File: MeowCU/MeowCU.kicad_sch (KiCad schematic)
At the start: 66 parts, among them J1 SWD, J10 Screw_Terminal_01x03, J11 Conn_02x10_Odd_Even, J2 Conn_02x04_Odd_Even, J4 SPI1, J5 5V_IN, J6 OLED, J7 USB_C_Receptacle_USB2.0_16P, J9 PWM, SW1 SW_SPST, SW6 BTN_UTIL, SW8 BTN_UTIL, SW9 BTN_UTIL, U1 STM32F405RGT6, U2 USBLC6-2SC6, U3 SN65HVD230, U4 AP2112K-3.3, Y1 25MHz

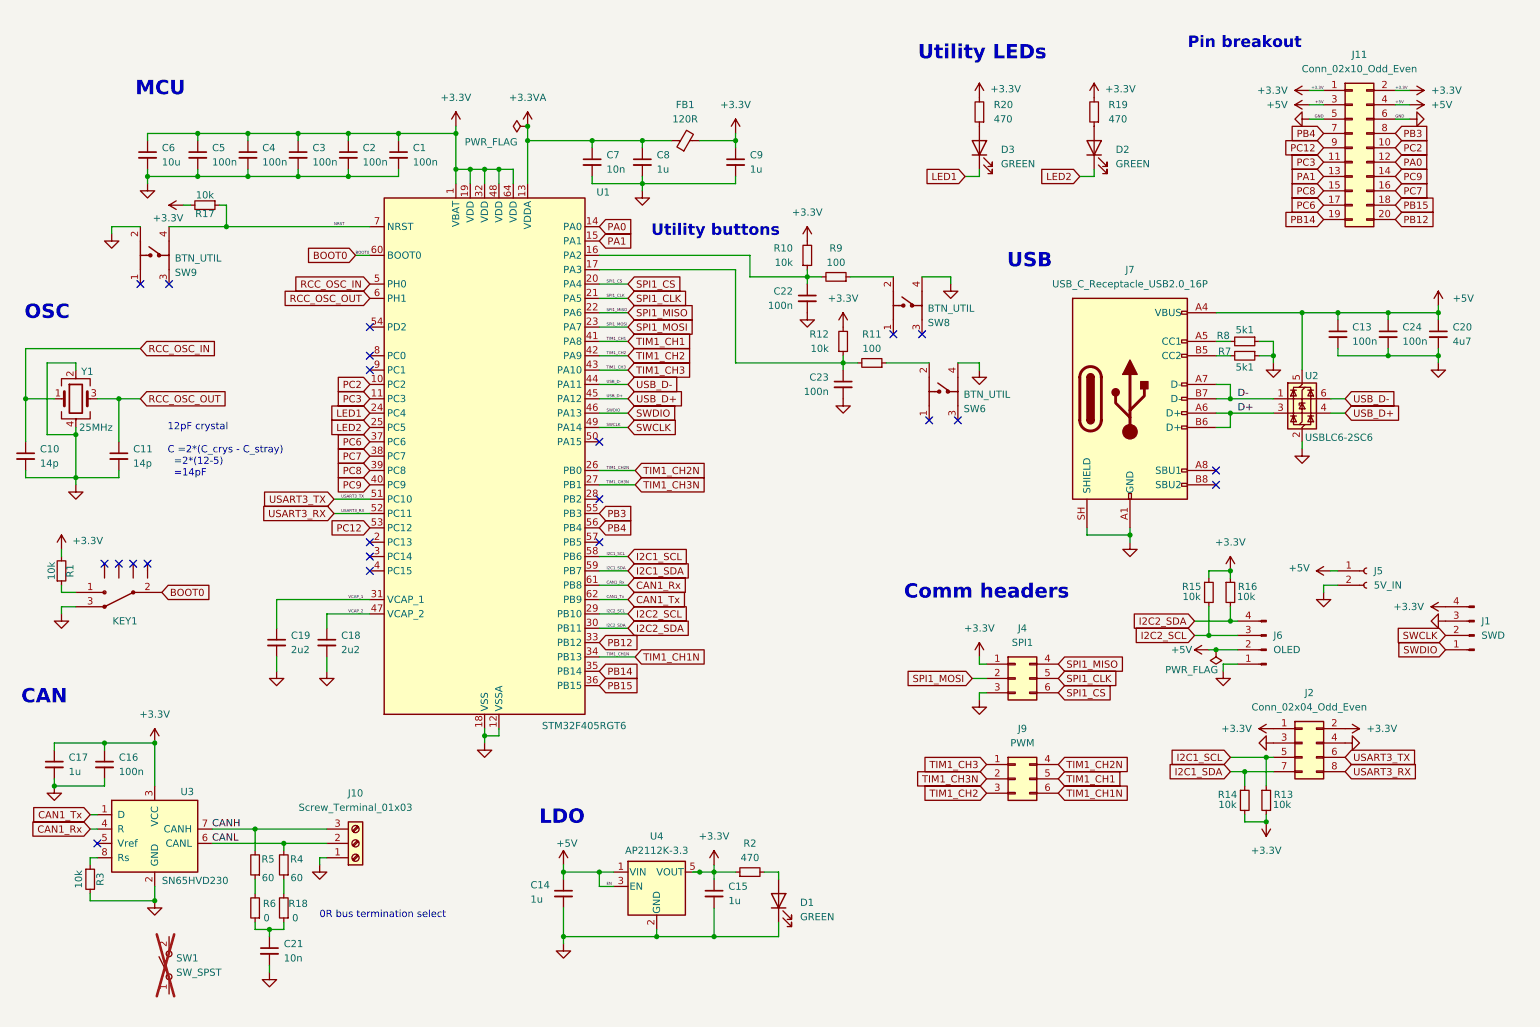
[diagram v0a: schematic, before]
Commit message: V1.7 Release
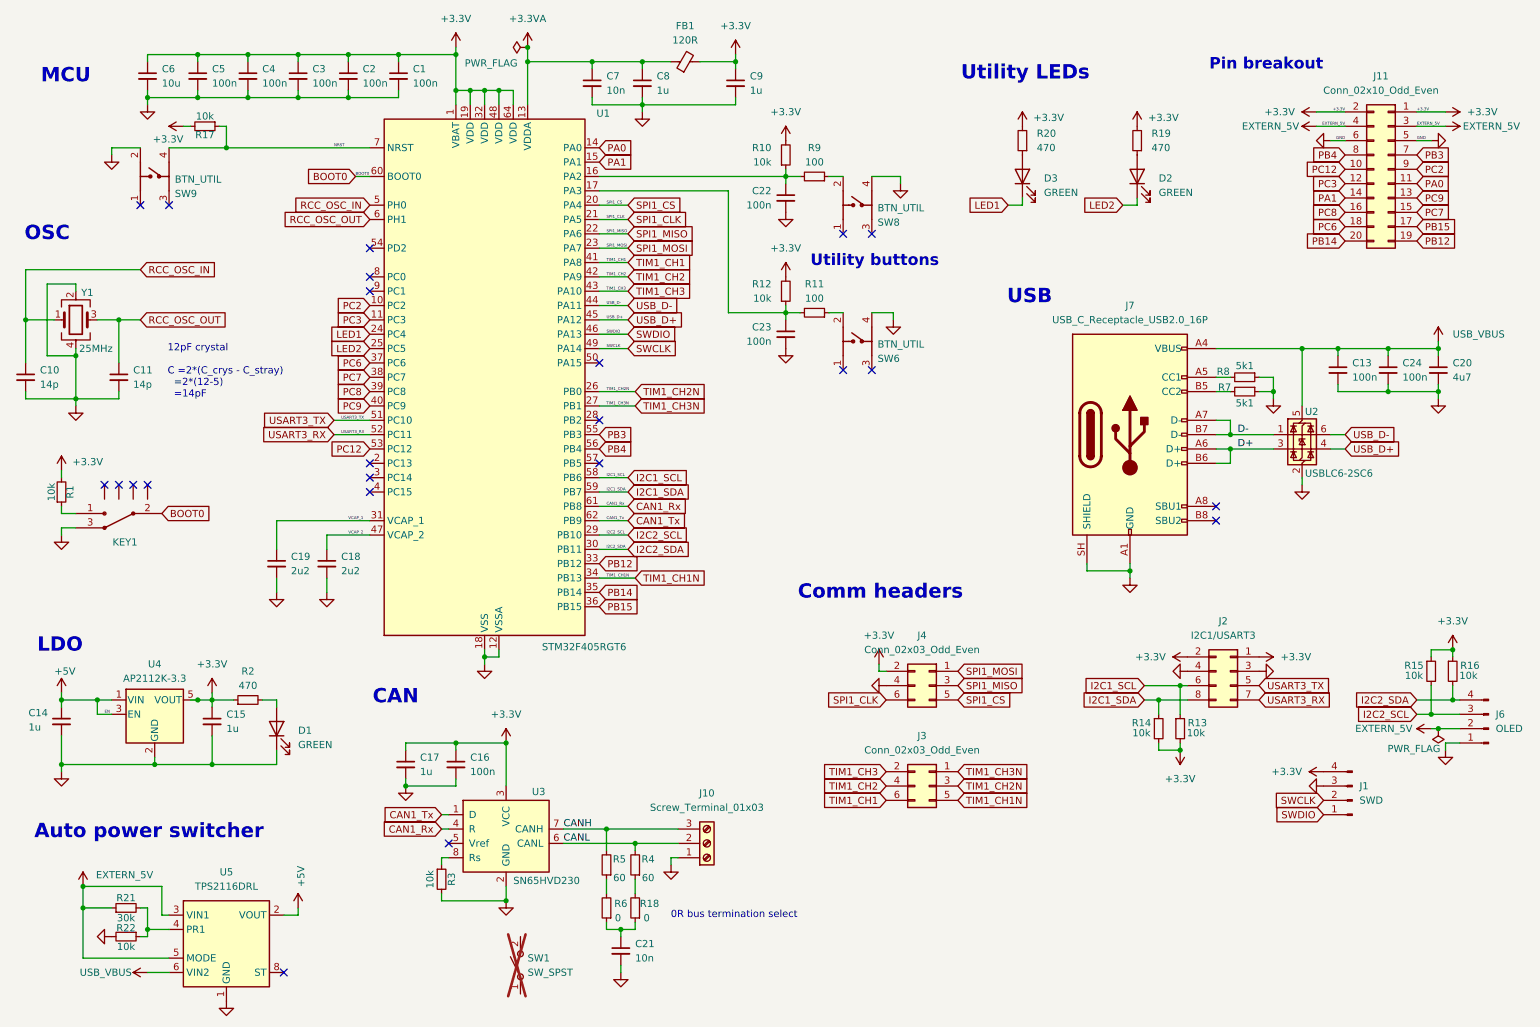
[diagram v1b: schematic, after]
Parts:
- removed J4: SPI1, Connector_PinHeader_2.54mm:PinHeader_2x03_P2.54mm_Vertical, symbol Connector_Generic:Conn_02x03_Top_Bottom
- removed J5: 5V_IN, Connector_PinHeader_2.54mm:PinHeader_1x02_P2.54mm_Vertical, symbol Connector:Conn_01x02_Socket
- removed J9: PWM, Connector_PinHeader_2.54mm:PinHeader_2x03_P2.54mm_Vertical, symbol Connector_Generic:Conn_02x03_Top_Bottom
- added J3, J4: Conn_02x03_Odd_Even, Connector_PinSocket_2.54mm:PinSocket_2x03_P2.54mm_Vertical, symbol Connector_Generic:Conn_02x03_Odd_Even
- added R21: 30k, Resistor_SMD:R_0402_1005Metric, symbol Device:R_Small
- added R22: 10k, Resistor_SMD:R_0402_1005Metric, symbol Device:R_Small
- added U5: TPS2116DRL, Package_TO_SOT_SMD:SOT-583-8, symbol Power_Management:TPS2116DRL
- J11: footprint Connector_PinHeader_2.54mm:PinHeader_2x10_P2.54mm_Vertical -> Connector_PinSocket_2.54mm:PinSocket_2x10_P2.54mm_Vertical
- J2: value Conn_02x04_Odd_Even -> I2C1/USART3; footprint Connector_PinHeader_2.54mm:PinHeader_2x04_P2.54mm_Vertical -> Connector_PinSocket_2.54mm:PinSocket_2x04_P2.54mm_Vertical
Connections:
- net +3.3V: now also J4.2 (Pin_2)
- net +5V: now also U5.2 (VOUT), U5.7 (VOUT); no longer C13.1, C20.1, C24.1, J11.3 (Pin_3), J11.4 (Pin_4), J6.2 (Pin_2), J7.A4 (VBUS), J7.A9 (VBUS), J7.B4 (VBUS), J7.B9 (VBUS), U2.5 (VBUS)
- net GND: now also J4.4 (Pin_4), R22.2, U5.1 (GND)
- net I2C1_SCL: now also J2.6 (Pin_6); no longer J2.5 (Pin_5)
- net I2C1_SDA: now also J2.8 (Pin_8); no longer J2.7 (Pin_7)
- net PA0: now also J11.11 (Pin_11); no longer J11.12 (Pin_12)
- net PA1: now also J11.14 (Pin_14); no longer J11.13 (Pin_13)
- net PB12: now also J11.19 (Pin_19); no longer J11.20 (Pin_20)
- net PB14: now also J11.20 (Pin_20); no longer J11.19 (Pin_19)
- net PB15: now also J11.17 (Pin_17); no longer J11.18 (Pin_18)
- net PB3: now also J11.7 (Pin_7); no longer J11.8 (Pin_8)
- net PB4: now also J11.8 (Pin_8); no longer J11.7 (Pin_7)
- net PC12: now also J11.10 (Pin_10); no longer J11.9 (Pin_9)
- net PC2: now also J11.9 (Pin_9); no longer J11.10 (Pin_10)
- net PC3: now also J11.12 (Pin_12); no longer J11.11 (Pin_11)
- net PC6: now also J11.18 (Pin_18); no longer J11.17 (Pin_17)
- net PC7: now also J11.15 (Pin_15); no longer J11.16 (Pin_16)
- net PC8: now also J11.16 (Pin_16); no longer J11.15 (Pin_15)
- net PC9: now also J11.13 (Pin_13); no longer J11.14 (Pin_14)
- net SPI1_CLK: now also J4.6 (Pin_6)
- net SPI1_CS: now also J4.5 (Pin_5)
- net SPI1_MISO: now also J4.3 (Pin_3)
- net SPI1_MOSI: now also J4.1 (Pin_1)
- net TIM1_CH1: now also J3.6 (Pin_6)
- net TIM1_CH1N: now also J3.5 (Pin_5)
- net TIM1_CH2: now also J3.4 (Pin_4)
- net TIM1_CH2N: now also J3.3 (Pin_3)
- net TIM1_CH3: now also J3.2 (Pin_2)
- net TIM1_CH3N: now also J3.1 (Pin_1)
- net USART3_RX: now also J2.7 (Pin_7); no longer J2.8 (Pin_8)
- net USART3_TX: now also J2.5 (Pin_5); no longer J2.6 (Pin_6)
- new net: R21.2, R22.1, U5.4 (PR1)
- new net EXTERN_5V: J11.3 (Pin_3), J11.4 (Pin_4), J6.2 (Pin_2), R21.1, U5.3 (VIN1), U5.5 (MODE)
- new net USB_VBUS: C13.1, C20.1, C24.1, J7.A4 (VBUS), J7.A9 (VBUS), J7.B4 (VBUS), J7.B9 (VBUS), U2.5 (VBUS), U5.6 (VIN2)
- no-connect marks 22 -> 23
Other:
- note added: "Auto power switcher"
- moved on the sheet: C1, C10, C11, C13, C14, C15, C16, C17, C18, C19, C2, C20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
